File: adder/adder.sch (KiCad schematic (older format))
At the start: 1 part, among them U1 mini-vertical-slide-switch

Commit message: First (incomplete) version of a 4-bit adder
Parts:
- added D1, D2, D3, D4: LED, symbol LED
- added J1: CONN_01X02, library:screw-terminal-01x02, symbol CONN_01X02
- added U10, U2: XOR, symbol so14
- added U11, U3: AND, symbol so14
- added U12, U13, U4, U5, U6, U8, U9: mini-vertical-slide-switch, library:mini-vertical-slide-switch, symbol mini-vertical-slide-switch
- added U7: OR, symbol so14
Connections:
- net labels added: A1, A2, A3, A4, AI2, AI3, AI4, B1, B2, B3, B4, C1, C2, C3, C4, CA2, CA3, CA4, GND, S1, S2, S3, S4, VCC, XI2, XI3, XI4
- wire segments 0 -> 150
- no-connect marks 0 -> 17

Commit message: Finished diagram and started on pcb layout hell
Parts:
- removed J1: CONN_01X02, library:screw-terminal-01x02, symbol CONN_01X02
- removed U1: mini-vertical-slide-switch, library:mini-vertical-slide-switch, symbol mini-vertical-slide-switch
- removed U3: AND, symbol so14
- added D10: LB4, LEDs:LED_0805_HandSoldering, symbol LED
- added D11: A4, LEDs:LED_0805_HandSoldering, symbol LED
- added D12: S4, LEDs:LED_0805_HandSoldering, symbol LED
- added D5: LB2, LEDs:LED_0805_HandSoldering, symbol LED
- added D6: LA2, LEDs:LED_0805_HandSoldering, symbol LED
- added D7: LB3, LEDs:LED_0805_HandSoldering, symbol LED
- added D8: LA3, LEDs:LED_0805_HandSoldering, symbol LED
- added D9: S3, LEDs:LED_0805_HandSoldering, symbol LED
- added J1: VIN, Pin_Headers:Pin_Header_Straight_1x03_Pitch2.54mm, symbol Conn_01x03
- added J2: B, Pin_Headers:Pin_Header_Straight_1x04_Pitch2.54mm, symbol Conn_01x04
- added J3: A, Pin_Headers:Pin_Header_Straight_1x04_Pitch2.54mm, symbol Conn_01x04
- added J4: VOUT, Pin_Headers:Pin_Header_Straight_1x03_Pitch2.54mm, symbol Conn_01x03
- added U1: XOR, library:ssop14, symbol so14
- added U3: A1, library:mini-vertical-slide-switch, symbol mini-vertical-slide-switch
- D1: value LED -> S1; footprint (none) -> LEDs:LED_0805_HandSoldering
- D2: value LED -> LB1; footprint (none) -> LEDs:LED_0805_HandSoldering
- D3: value LED -> LA1; footprint (none) -> LEDs:LED_0805_HandSoldering
- D4: value LED -> S2; footprint (none) -> LEDs:LED_0805_HandSoldering
- U10, U11, U7: footprint (none) -> library:ssop14
- U12: value mini-vertical-slide-switch -> A4
- U13: value mini-vertical-slide-switch -> B4
- U2: value XOR -> AND; footprint (none) -> library:ssop14
- U4: value mini-vertical-slide-switch -> B1
- U5: value mini-vertical-slide-switch -> A2
- U6: value mini-vertical-slide-switch -> B2
- U8: value mini-vertical-slide-switch -> A3
- U9: value mini-vertical-slide-switch -> B3
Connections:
- net labels added: AI1, CIN, COUT, CX1, CX2, CX3, CX4, VOUT, XI1
- net labels removed: C4, CA2, CA3, CA4
- wire segments 150 -> 198
- no-connect marks 17 -> 8

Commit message: Finished v2 of adder
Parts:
- U12, U13, U3, U4, U5, U6, U8, U9: symbol mini-vertical-slide-switch -> mini-vertical-slide-switch-RESCUE-adder
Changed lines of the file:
@@
 EESchema Schematic File Version 2
+LIBS:adder-rescue
 LIBS:power
 LIBS:device
@@
 $EndDescr
 $Comp
-L mini-vertical-slide-switch U3
+L mini-vertical-slide-switch-RESCUE-adder U3
 U 1 1 5A8D4725
 P 3350 1450
@@
 NoConn ~ 3200 1750
 $Comp
-L mini-vertical-slide-switch U5
+L mini-vertical-slide-switch-RESCUE-adder U5
 U 1 1 5A8D472D
 P 5050 1450
@@
 NoConn ~ 4900 1750
 $Comp
-L mini-vertical-slide-switch U8
+L mini-vertical-slide-switch-RESCUE-adder U8
 U 1 1 5A8D4735
 P 6750 1400
@@
 NoConn ~ 6600 1700
 $Comp
-L mini-vertical-slide-switch U12
+L mini-vertical-slide-switch-RESCUE-adder U12
 U 1 1 5A8D473D
 P 8450 1400
@@
 	8600 1700 8600 2250
 $Comp
-L mini-vertical-slide-switch U4
+L mini-vertical-slide-switch-RESCUE-adder U4
 U 1 1 5A8D4839
 P 3400 6450
@@
 NoConn ~ 3550 6150
 $Comp
-L mini-vertical-slide-switch U6
+L mini-vertical-slide-switch-RESCUE-adder U6
 U 1 1 5A8D4847
 P 5350 6450
@@
 NoConn ~ 5500 6150
 $Comp
-L mini-vertical-slide-switch U9
+L mini-vertical-slide-switch-RESCUE-adder U9
 U 1 1 5A8D4855
 P 6850 6450
@@
 NoConn ~ 7000 6150
 $Comp
-L mini-vertical-slide-switch U13
+L mini-vertical-slide-switch-RESCUE-adder U13
 U 1 1 5A8D4863
 P 8800 6450

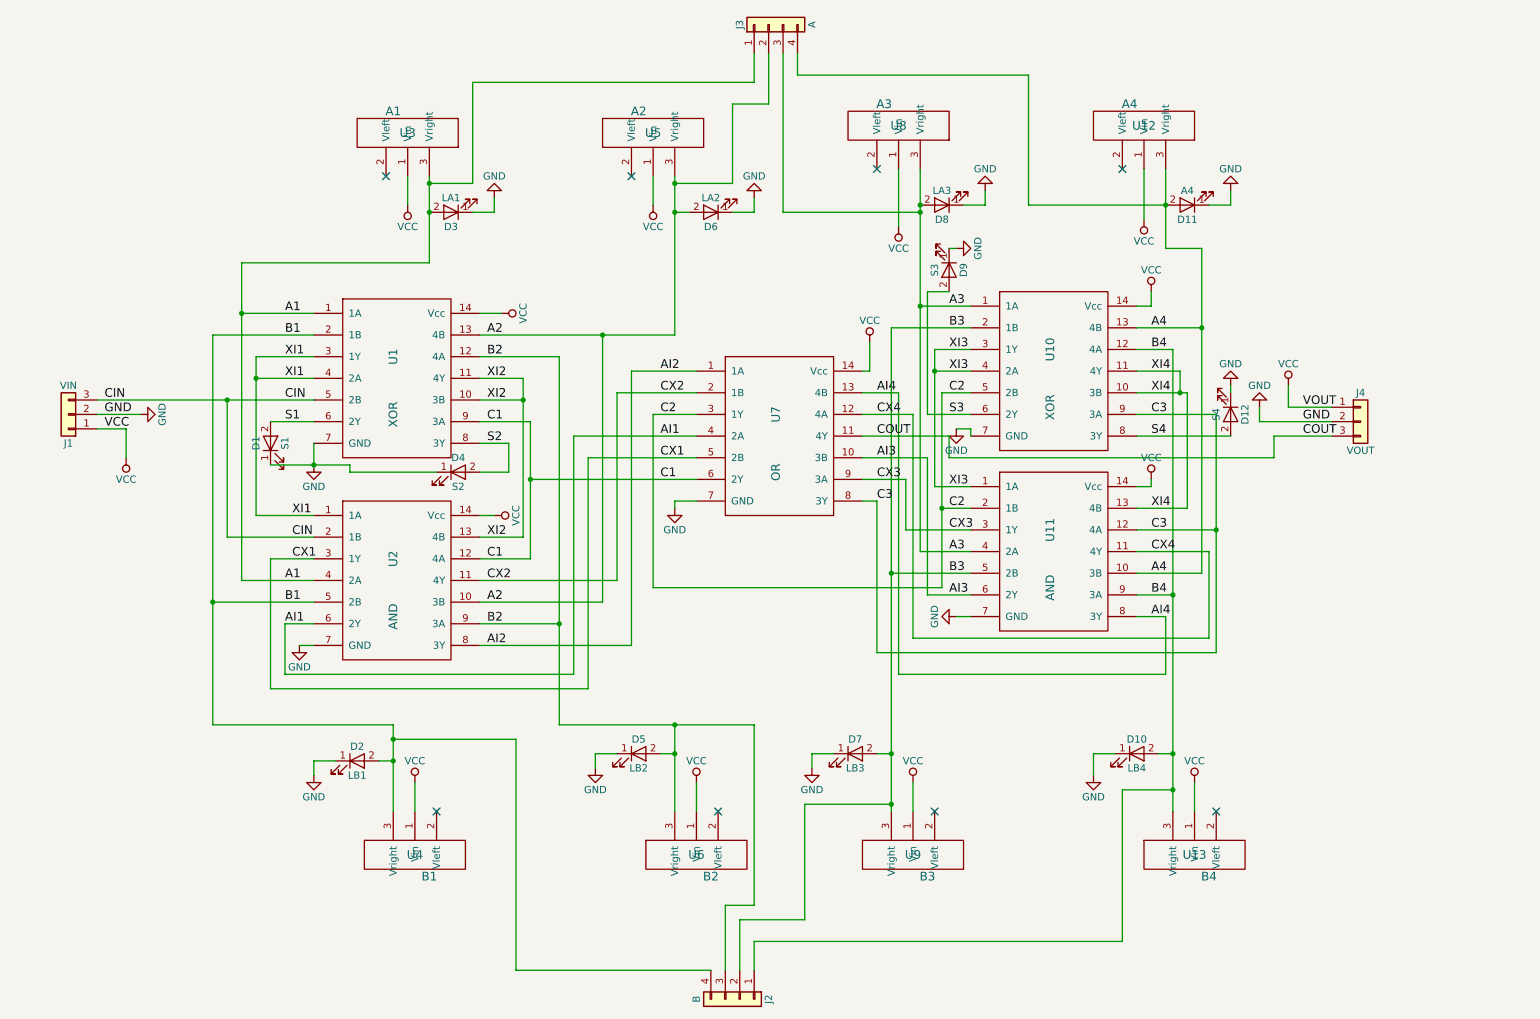
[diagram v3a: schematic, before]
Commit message: Started on adder v3
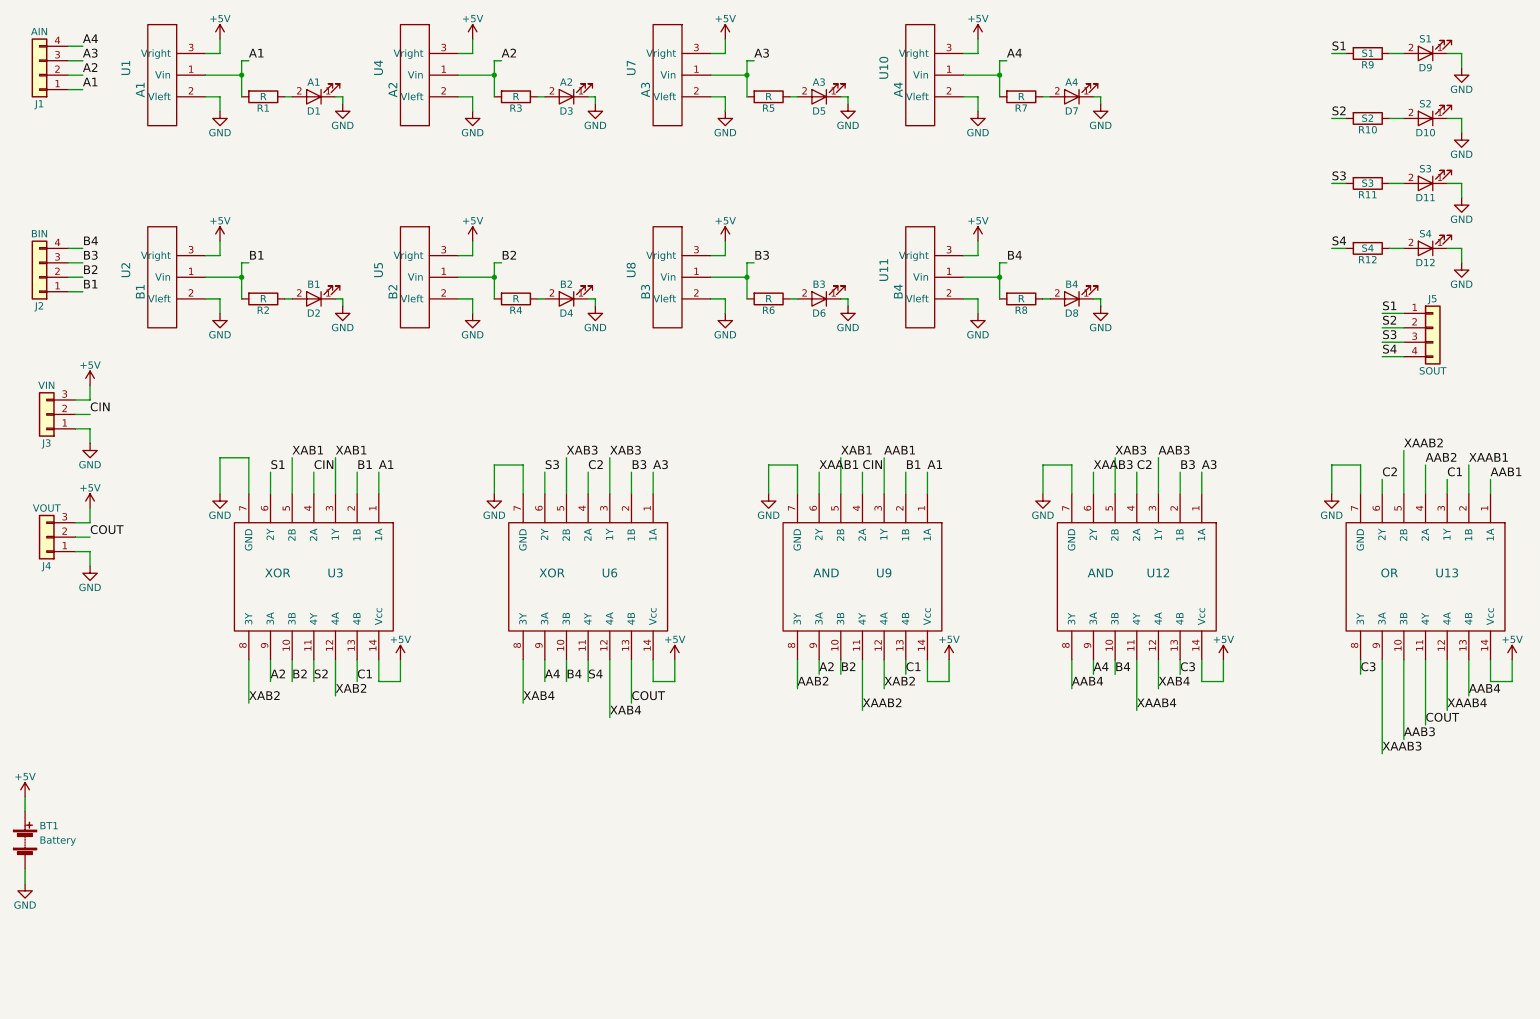
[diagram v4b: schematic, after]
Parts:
- removed J1: VIN, Pin_Headers:Pin_Header_Straight_1x03_Pitch2.54mm, symbol Conn_01x03
- removed J3: A, Pin_Headers:Pin_Header_Straight_1x04_Pitch2.54mm, symbol Conn_01x04
- removed U1, U10: XOR, library:ssop14, symbol so14
- removed U11, U2: AND, library:ssop14, symbol so14
- removed U12: A4, library:mini-vertical-slide-switch, symbol mini-vertical-slide-switch-RESCUE-adder
- removed U13: B4, library:mini-vertical-slide-switch, symbol mini-vertical-slide-switch-RESCUE-adder
- removed U3: A1, library:mini-vertical-slide-switch, symbol mini-vertical-slide-switch-RESCUE-adder
- removed U4: B1, library:mini-vertical-slide-switch, symbol mini-vertical-slide-switch-RESCUE-adder
- removed U5: A2, library:mini-vertical-slide-switch, symbol mini-vertical-slide-switch-RESCUE-adder
- removed U6: B2, library:mini-vertical-slide-switch, symbol mini-vertical-slide-switch-RESCUE-adder
- removed U7: OR, library:ssop14, symbol so14
- removed U8: A3, library:mini-vertical-slide-switch, symbol mini-vertical-slide-switch-RESCUE-adder
- removed U9: B3, library:mini-vertical-slide-switch, symbol mini-vertical-slide-switch-RESCUE-adder
- added BT1: Battery, Air_Coils_SML_NEOSID:Neosid_Air-Coil_SML_1turn_HDM0131A, symbol Battery
- added J1: AIN, Socket_Strips:Socket_Strip_Straight_1x04_Pitch2.54mm, symbol Conn_01x04
- added J3: VIN, Socket_Strips:Socket_Strip_Straight_1x03_Pitch2.54mm, symbol Conn_01x03
- added J5: SOUT, Socket_Strips:Socket_Strip_Straight_1x04_Pitch2.54mm, symbol Conn_01x04
- added R1, R2, R3, R4, R5, R6, R7, R8: R, Resistors_SMD:R_0805_HandSoldering, symbol R
- added R10: S2, Resistors_SMD:R_0805_HandSoldering, symbol R
- added R11: S3, Resistors_SMD:R_0805_HandSoldering, symbol R
- added R12: S4, Resistors_SMD:R_0805_HandSoldering, symbol R
- added R9: S1, Resistors_SMD:R_0805_HandSoldering, symbol R
- added U1: A1, library:mini-vertical-slide-switch, symbol mini-vertical-slide-switch
- added U10: A4, library:mini-vertical-slide-switch, symbol mini-vertical-slide-switch
- added U11: B4, library:mini-vertical-slide-switch, symbol mini-vertical-slide-switch
- added U12, U9: AND, library:ssop14, symbol so14
- added U13: OR, library:ssop14, symbol so14
- added U2: B1, library:mini-vertical-slide-switch, symbol mini-vertical-slide-switch
- added U3, U6: XOR, library:ssop14, symbol so14
- added U4: A2, library:mini-vertical-slide-switch, symbol mini-vertical-slide-switch
- added U5: B2, library:mini-vertical-slide-switch, symbol mini-vertical-slide-switch
- added U7: A3, library:mini-vertical-slide-switch, symbol mini-vertical-slide-switch
- added U8: B3, library:mini-vertical-slide-switch, symbol mini-vertical-slide-switch
- D1: value S1 -> A1
- D10: value LB4 -> S2
- D11: value A4 -> S3
- D2: value LB1 -> B1
- D3: value LA1 -> A2
- D4: value S2 -> B2
- D5: value LB2 -> A3
- D6: value LA2 -> B3
- D7: value LB3 -> A4
- D8: value LA3 -> B4
- D9: value S3 -> S1
- J2: value B -> BIN; footprint Pin_Headers:Pin_Header_Straight_1x04_Pitch2.54mm -> Socket_Strips:Socket_Strip_Straight_1x04_Pitch2.54mm
- J4: footprint Pin_Headers:Pin_Header_Straight_1x03_Pitch2.54mm -> Socket_Strips:Socket_Strip_Straight_1x03_Pitch2.54mm
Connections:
- net VCC is gone; now on net GND: J4.1 (Pin_1)
- net A1: now also J1.1 (Pin_1), R1.2, U1.1 (Vin), U3.1 (1A), U9.1 (1A); no longer D3.2 (A)
- net A2: now also J1.2 (Pin_2), R3.2, U3.9 (3A), U4.1 (Vin), U9.9 (3A); no longer D6.2 (A)
- net A3: now also J1.3 (Pin_3), R5.2, U12.1 (1A), U6.1 (1A), U7.1 (Vin); no longer D8.2 (A)
- net A4: now also J1.4 (Pin_4), R7.2, U10.1 (Vin), U12.9 (3A), U6.9 (3A); no longer D11.2 (A)
- net B1: now also J2.1 (Pin_1), R2.2, U2.1 (Vin), U3.2 (1B), U9.2 (1B); no longer D2.2 (A), J2.4 (Pin_4)
- net B2: now also J2.2 (Pin_2), R4.2, U3.10 (3B), U5.1 (Vin), U9.10 (3B); no longer D5.2 (A), J2.3 (Pin_3)
- net B3: now also J2.3 (Pin_3), R6.2, U12.2 (1B), U6.2 (1B), U8.1 (Vin); no longer D7.2 (A), J2.2 (Pin_2)
- net B4: now also J2.4 (Pin_4), R8.2, U11.1 (Vin), U12.10 (3B), U6.10 (3B); no longer D10.2 (A), J2.1 (Pin_1)
- net C1: now also U13.3 (1Y), U3.13 (4B), U9.13 (4B)
- net C2: now also U12.4 (2A), U13.6 (2Y), U6.4 (2A)
- net C3: now also U12.13 (4B), U13.8 (3Y)
- net CIN: now also J3.2 (Pin_2), U3.4 (2A), U9.4 (2A)
- net COUT: now also J4.2 (Pin_2), U13.11 (4Y), U6.13 (4B); no longer J4.3 (Pin_3)
- net GND: now also BT1.2 (-), J3.1 (Pin_1), U1.2 (Vleft), U10.2 (Vleft), U11.2 (Vleft), U12.7 (GND), U13.7 (GND), U2.2 (Vleft), U3.7 (GND), U4.2 (Vleft), U5.2 (Vleft), U6.7 (GND), U7.2 (Vleft), U8.2 (Vleft), U9.7 (GND); no longer J4.2 (Pin_2)
- net S1: now also J5.1 (Pin_1), R9.2, U3.6 (2Y); no longer D1.2 (A)
- net S2: now also J5.2 (Pin_2), R10.2, U3.11 (4Y); no longer D4.2 (A)
- net S3: now also J5.3 (Pin_3), R11.2, U6.6 (2Y); no longer D9.2 (A)
- net S4: now also J5.4 (Pin_4), R12.2, U6.11 (4Y); no longer D12.2 (A)
- new net: D1.2 (A), R1.1
- new net: D3.2 (A), R3.1
- new net: D5.2 (A), R5.1
- new net: D7.2 (A), R7.1
- new net: D2.2 (A), R2.1
- new net: D4.2 (A), R4.1
- new net: D6.2 (A), R6.1
- new net: D8.2 (A), R8.1
- new net: D9.2 (A), R9.1
- new net: D10.2 (A), R10.1
- new net: D11.2 (A), R11.1
- new net: D12.2 (A), R12.1
- new net +5V: BT1.1 (+), J3.3 (Pin_3), J4.3 (Pin_3), U1.3 (Vright), U10.3 (Vright), U11.3 (Vright), U12.14 (Vcc), U13.14 (Vcc), U2.3 (Vright), U3.14 (Vcc), U4.3 (Vright), U5.3 (Vright), U6.14 (Vcc), U7.3 (Vright), U8.3 (Vright), U9.14 (Vcc)
- new net AAB1: U13.1 (1A), U9.3 (1Y)
- new net AAB2: U13.4 (2A), U9.8 (3Y)
- new net AAB3: U12.3 (1Y), U13.10 (3B)
- new net AAB4: U12.8 (3Y), U13.13 (4B)
- new net XAAB1: U13.2 (1B), U9.6 (2Y)
- new net XAAB2: U13.5 (2B), U9.11 (4Y)
- new net XAAB3: U12.6 (2Y), U13.9 (3A)
- new net XAAB4: U12.11 (4Y), U13.12 (4A)
- new net XAB1: U3.3 (1Y), U3.5 (2B), U9.5 (2B)
- new net XAB2: U3.12 (4A), U3.8 (3Y), U9.12 (4A)
- new net XAB3: U12.5 (2B), U6.3 (1Y), U6.5 (2B)
- new net XAB4: U12.12 (4A), U6.12 (4A), U6.8 (3Y)
- no-connect marks 8 -> 0
